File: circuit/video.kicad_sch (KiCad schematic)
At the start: 4 parts, among them J1 Port B, J2 Port C, J4 Port A, J4 Port G

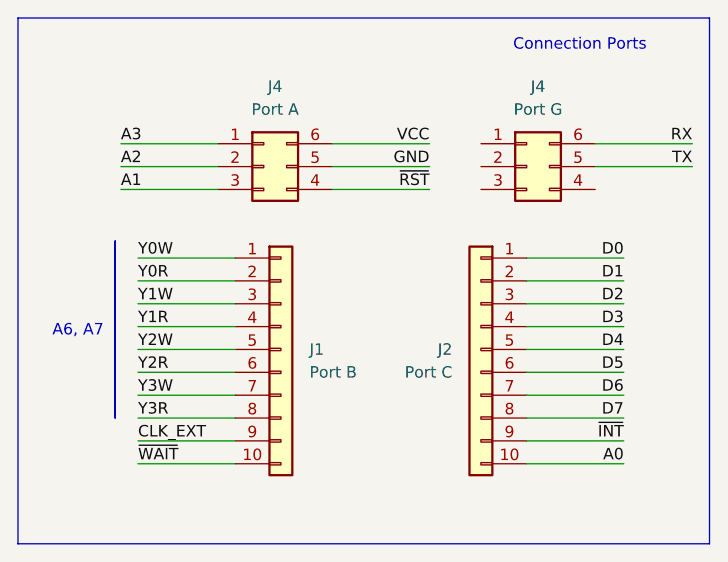
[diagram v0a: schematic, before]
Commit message: .
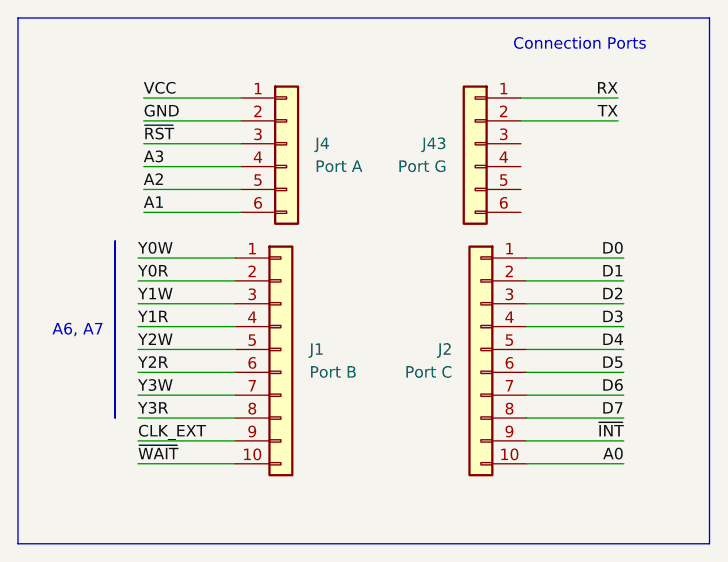
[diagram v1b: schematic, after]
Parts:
- removed J4: Port A, symbol Connector_Generic:Conn_02x03_Counter_Clockwise
- removed J4: Port G, symbol Connector_Generic:Conn_02x03_Counter_Clockwise
- added J4: Port A, symbol Connector_Generic:Conn_01x06
- added J43: Port G, symbol Connector_Generic:Conn_01x06
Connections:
- net A1: now also J4.6 (Pin_6)
- net A2: now also J4.5 (Pin_5)
- net A3: now also J4.4 (Pin_4)
- net GND: now also J4.2 (Pin_2)
- net RX: now also J43.1 (Pin_1)
- net TX: now also J43.2 (Pin_2)
- net VCC: now also J4.1 (Pin_1)
- net ~{RST}: now also J4.3 (Pin_3)
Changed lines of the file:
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@@
 (kicad_sch (version 20230121) (generator eeschema)
   (paper "A4")
+  (wire (pts (xy 216.535 31.75) (xy 227.33 31.75))
+    (stroke (width 0) (type default))
+  )
+  (wire (pts (xy 216.535 39.37) (xy 227.33 39.37))
+    (stroke (width 0) (type default))
+  )
   (wire (pts (xy 269.875 62.23) (xy 259.08 62.23))
     (stroke (width 0) (type default))
   )
-  (wire (pts (xy 277.495 34.29) (xy 266.7 34.29))
+  (wire (pts (xy 216.535 36.83) (xy 227.33 36.83))
+    (stroke (width 0) (type default))
+  )
+  (wire (pts (xy 269.24 26.67) (xy 258.445 26.67))
     (stroke (width 0) (type default))
   )
@@
     (stroke (width 0) (type default))
   )
-  (wire (pts (xy 248.285 36.83) (xy 237.49 36.83))
-    (stroke (width 0) (type default))
-  )
   (wire (pts (xy 269.875 44.45) (xy 259.08 44.45))
     (stroke (width 0) (type default))
@@
     (stroke (width 0) (type default))
   )
-  (wire (pts (xy 277.495 31.75) (xy 266.7 31.75))
-    (stroke (width 0) (type default))
-  )
   (wire (pts (xy 215.9 62.23) (xy 226.695 62.23))
     (stroke (width 0) (type default))
@@
     (stroke (width 0) (type default))
   )
-  (wire (pts (xy 213.995 36.83) (xy 224.79 36.83))
-    (stroke (width 0) (type default))
-  )
   (wire (pts (xy 215.9 54.61) (xy 226.695 54.61))
     (stroke (width 0) (type default))
@@
     (stroke (width 0) (type default))
   )
-  (wire (pts (xy 213.995 34.29) (xy 224.79 34.29))
+  (wire (pts (xy 216.535 34.29) (xy 227.33 34.29))
+    (stroke (width 0) (type default))
+  )
+  (wire (pts (xy 269.24 29.21) (xy 258.445 29.21))
+    (stroke (width 0) (type default))
+  )
+  (wire (pts (xy 216.535 26.67) (xy 227.33 26.67))
     (stroke (width 0) (type default))
   )
@@
     (stroke (width 0) (type default))
   )
+  (wire (pts (xy 216.535 29.21) (xy 227.33 29.21))
+    (stroke (width 0) (type default))
+  )
   (wire (pts (xy 215.9 67.31) (xy 226.695 67.31))
     (stroke (width 0) (type default))
   )
-  (wire (pts (xy 248.285 34.29) (xy 237.49 34.29))
-    (stroke (width 0) (type default))
-  )
-  (wire (pts (xy 248.285 31.75) (xy 237.49 31.75))
-    (stroke (width 0) (type default))
-  )
   (wire (pts (xy 215.9 44.45) (xy 226.695 44.45))
     (stroke (width 0) (type default))
   )
-  (wire (pts (xy 213.995 31.75) (xy 224.79 31.75))
-    (stroke (width 0) (type default))
-  )
   (rectangle (start 213.36 42.545) (end 213.36 62.23)
     (stroke (width 0) (type default))
@@
     (effects (font (size 1.27 1.27)) (justify right bottom))
   )
-  (label "A1" (at 213.995 36.83 0) (fields_autoplaced)
-    (effects (font (size 1.27 1.27)) (justify left bottom))
-  )
   (label "Y1W" (at 215.9 49.53 0) (fields_autoplaced)
     (effects (font (size 1.27 1.27)) (justify left bottom))
@@
     (effects (font (size 1.27 1.27)) (justify right bottom))
   )
-  (label "A2" (at 213.995 34.29 0) (fields_autoplaced)
-    (effects (font (size 1.27 1.27)) (justify left bottom))
-  )
-  (label "A3" (at 213.995 31.75 0) (fields_autoplaced)
-    (effects (font (size 1.27 1.27)) (justify left bottom))
-  )
   (label "Y3W" (at 215.9 59.69 0) (fields_autoplaced)
     (effects (font (size 1.27 1.27)) (justify left bottom))
   )
+  (label "A1" (at 216.535 39.37 0) (fields_autoplaced)
+    (effects (font (size 1.27 1.27)) (justify left bottom))
+  )
+  (label "A3" (at 216.535 34.29 0) (fields_autoplaced)
+    (effects (font (size 1.27 1.27)) (justify left bottom))
+  )
   (label "~{WAIT}" (at 215.9 67.31 0) (fields_autoplaced)
     (effects (font (size 1.27 1.27)) (justify left bottom))
   )
-  (label "GND" (at 248.285 34.29 180) (fields_autoplaced)
-    (effects (font (size 1.27 1.27)) (justify right bottom))
-  )
-  (label "~{RST}" (at 248.285 36.83 180) (fields_autoplaced)
+  (label "VCC" (at 216.535 26.67 0) (fields_autoplaced)
+    (effects (font (size 1.27 1.27)) (justify left bottom))
+  )
+  (label "GND" (at 216.535 29.21 0) (fields_autoplaced)
+    (effects (font (size 1.27 1.27)) (justify left bottom))
+  )
+  (label "RX" (at 269.24 26.67 180) (fields_autoplaced)
     (effects (font (size 1.27 1.27)) (justify right bottom))
   )
@@
     (effects (font (size 1.27 1.27)) (justify right bottom))
   )
-  (label "RX" (at 277.495 31.75 180) (fields_autoplaced)
-    (effects (font (size 1.27 1.27)) (justify right bottom))
-  )
   (label "Y0W" (at 215.9 44.45 0) (fields_autoplaced)
     (effects (font (size 1.27 1.27)) (justify left bottom))
@@
     (effects (font (size 1.27 1.27)) (justify right bottom))
   )
+  (label "TX" (at 269.24 29.21 180) (fields_autoplaced)
+    (effects (font (size 1.27 1.27)) (justify right bottom))
+  )
   (label "Y0R" (at 215.9 46.99 0) (fields_autoplaced)
     (effects (font (size 1.27 1.27)) (justify left bottom))
@@
     (effects (font (size 1.27 1.27)) (justify left bottom))
   )
-  (label "VCC" (at 248.285 31.75 180) (fields_autoplaced)
-    (effects (font (size 1.27 1.27)) (justify right bottom))
-  )
-  (label "TX" (at 277.495 34.29 180) (fields_autoplaced)
-    (effects (font (size 1.27 1.27)) (justify right bottom))
+  (label "A2" (at 216.535 36.83 0) (fields_autoplaced)
+    (effects (font (size 1.27 1.27)) (justify left bottom))
   )
   (label "Y2W" (at 215.9 54.61 0) (fields_autoplaced)
@@
     (effects (font (size 1.27 1.27)) (justify right bottom))
   )
+  (label "~{RST}" (at 216.535 31.75 0) (fields_autoplaced)
+    (effects (font (size 1.27 1.27)) (justify left bottom))
+  )
   (label "D2" (at 269.875 49.53 180) (fields_autoplaced)
     (effects (font (size 1.27 1.27)) (justify right bottom))
+  )
+  (symbol (lib_id "Connector_Generic:Conn_01x06") (at 253.365 31.75 0) (mirror y) (unit 1)
+    (in_bom yes) (on_board yes) (dnp no)
+    (property "Reference" "J43" (at 250.19 31.75 0)
+      (effects (font (size 1.27 1.27)) (justify left))
+    )
+    (property "Value" "Port G" (at 250.19 34.29 0)
+      (effects (font (size 1.27 1.27)) (justify left))
+    )
+    (property "Footprint" "" (at 253.365 31.75 0)
+      (effects (font (size 1.27 1.27)) hide)
+    )
+    (property "Datasheet" "~" (at 253.365 31.75 0)
+      (effects (font (size 1.27 1.27)) hide)
+    )
+    (pin "1")
+    (pin "2")
+    (pin "3")
+    (pin "4")
+    (pin "5")
+    (pin "6")
+    (instances
+      (project "fortuna-box"
+        (path "/0e4c4e8a-78e0-4f49-88dc-754c12656209"
+          (reference "J43") (unit 1)
+        )
+        (path "/0e4c4e8a-78e0-4f49-88dc-754c12656209/afd1b413-de30-4838-bb16-3d0c9f3cd196"
+          (reference "J33") (unit 1)
+        )
+        (path "/0e4c4e8a-78e0-4f49-88dc-754c12656209/7a4166e2-b1d1-4968-8160-8d4c6a581842"
+          (reference "J44") (unit 1)
+        )
+      )
+    )
   )
   (symbol (lib_id "Connector_Generic:Conn_01x10") (at 231.775 54.61 0) (unit 1)
@@
     )
   )
-  (symbol (lib_id "Connector_Generic:Conn_02x03_Counter_Clockwise") (at 229.87 34.29 0) (unit 1)
-    (in_bom yes) (on_board yes) (dnp no)
-    (property "Reference" "J4" (at 231.14 25.4 0)
-      (effects (font (size 1.27 1.27)))
-    )
-    (property "Value" "Port A" (at 231.14 27.94 0)
-      (effects (font (size 1.27 1.27)))
-    )
-    (property "Footprint" "" (at 229.87 34.29 0)
-      (effects (font (size 1.27 1.27)) hide)
-    )
-    (property "Datasheet" "~" (at 229.87 34.29 0)
-      (effects (font (size 1.27 1.27)) hide)
-    )
-    (pin "1")
-    (pin "2")
-    (pin "3")
-    (pin "4")
-    (pin "5")
-    (pin "6")
-    (instances
-      (project "fortuna-box"
-        (path "/0e4c4e8a-78e0-4f49-88dc-754c12656209"
-          (reference "J4") (unit 1)
-        )
-        (path "/0e4c4e8a-78e0-4f49-88dc-754c12656209/4037b4b4-0005-458e-a3e9-fe2ae826ab0c"
-          (reference "J19") (unit 1)
-        )
-        (path "/0e4c4e8a-78e0-4f49-88dc-754c12656209/0ad0c907-f2a9-47ff-aff1-7aaecbdef7ee"
-          (reference "J17") (unit 1)
-        )
-        (path "/0e4c4e8a-78e0-4f49-88dc-754c12656209/7a4166e2-b1d1-4968-8160-8d4c6a581842"
-          (reference "J38") (unit 1)
-        )
-      )
-    )
-  )
   (symbol (lib_id "Connector_Generic:Conn_01x10") (at 254 54.61 0) (mirror y) (unit 1)
     (in_bom yes) (on_board yes) (dnp no)
@@
     )
   )
-  (symbol (lib_id "Connector_Generic:Conn_02x03_Counter_Clockwise") (at 259.08 34.29 0) (unit 1)
-    (in_bom yes) (on_board yes) (dnp no)
-    (property "Reference" "J4" (at 260.35 25.4 0)
-      (effects (font (size 1.27 1.27)))
-    )
-    (property "Value" "Port G" (at 260.35 27.94 0)
-      (effects (font (size 1.27 1.27)))
-    )
-    (property "Footprint" "" (at 259.08 34.29 0)
-      (effects (font (size 1.27 1.27)) hide)
-    )
-    (property "Datasheet" "~" (at 259.08 34.29 0)
+  (symbol (lib_id "Connector_Generic:Conn_01x06") (at 232.41 31.75 0) (unit 1)
+    (in_bom yes) (on_board yes) (dnp no) (fields_autoplaced)
+    (property "Reference" "J4" (at 235.585 31.75 0)
+      (effects (font (size 1.27 1.27)) (justify left))
+    )
+    (property "Value" "Port A" (at 235.585 34.29 0)
+      (effects (font (size 1.27 1.27)) (justify left))
+    )
+    (property "Footprint" "" (at 232.41 31.75 0)
+      (effects (font (size 1.27 1.27)) hide)
+    )
+    (property "Datasheet" "~" (at 232.41 31.75 0)
       (effects (font (size 1.27 1.27)) hide)
     )
@@
         )
         (path "/0e4c4e8a-78e0-4f49-88dc-754c12656209/afd1b413-de30-4838-bb16-3d0c9f3cd196"
-          (reference "J33") (unit 1)
-        )
-        (path "/0e4c4e8a-78e0-4f49-88dc-754c12656209/4fe6965a-72a4-4531-8bd8-5a46765186a2"
-          (reference "J35") (unit 1)
-        )
-        (path "/0e4c4e8a-78e0-4f49-88dc-754c12656209/0ad0c907-f2a9-47ff-aff1-7aaecbdef7ee"
+          (reference "J7") (unit 1)
+        )
+        (path "/0e4c4e8a-78e0-4f49-88dc-754c12656209/7a4166e2-b1d1-4968-8160-8d4c6a581842"
           (reference "J37") (unit 1)
         )
-        (path "/0e4c4e8a-78e0-4f49-88dc-754c12656209/7a4166e2-b1d1-4968-8160-8d4c6a581842"
-          (reference "J41") (unit 1)
-        )
       )
